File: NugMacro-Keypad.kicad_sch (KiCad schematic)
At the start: 16 parts, among them J2 Conn_01x04, SW1 SW_Push, U1 ATmega32U4-A, Y1 16MHz

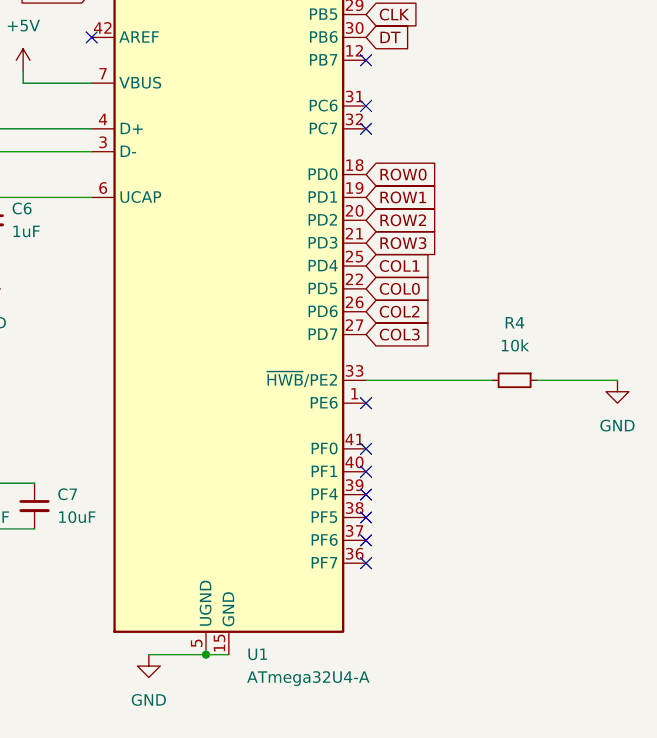
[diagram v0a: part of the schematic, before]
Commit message: First prototype pcb done
finally
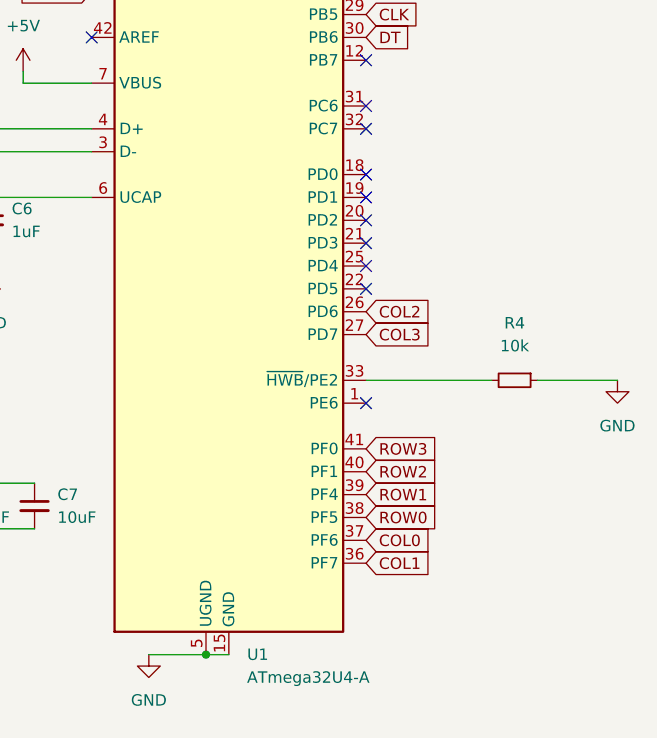
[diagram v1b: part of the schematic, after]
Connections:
- net COL0: now also U1.37 (PF6); no longer U1.22 (PD5)
- net COL1: now also U1.36 (PF7); no longer U1.25 (PD4)
- net ROW0: now also U1.38 (PF5); no longer U1.18 (PD0)
- net ROW1: now also U1.39 (PF4); no longer U1.19 (PD1)
- net ROW2: now also U1.40 (PF1); no longer U1.20 (PD2)
- net ROW3: now also U1.41 (PF0); no longer U1.21 (PD3)
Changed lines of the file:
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@@
   (no_connect (at 195.58 71.12))
   (no_connect (at 226.06 73.66))
-  (no_connect (at 226.06 124.46))
+  (no_connect (at 226.06 88.9))
+  (no_connect (at 226.06 86.36))
+  (no_connect (at 226.06 96.52))
   (no_connect (at 226.06 81.28))
-  (no_connect (at 226.06 119.38))
   (no_connect (at 226.06 111.76))
-  (no_connect (at 226.06 129.54))
   (no_connect (at 226.06 60.96))
+  (no_connect (at 226.06 93.98))
   (no_connect (at 226.06 63.5))
-  (no_connect (at 226.06 121.92))
-  (no_connect (at 226.06 127))
-  (no_connect (at 226.06 116.84))
+  (no_connect (at 226.06 91.44))
+  (no_connect (at 226.06 99.06))
   (no_connect (at 226.06 66.04))
   (no_connect (at 226.06 78.74))
@@
     )
   )
-  (global_label "ROW3" (shape input) (at 226.06 93.98 0) (fields_autoplaced)
-    (effects (font (size 1.27 1.27)) (justify left))
-    (property "Intersheet References" "${INTERSHEET_REFS}" (id 0) (at 233.7345 93.9006 0)
+  (global_label "ROW3" (shape input) (at 226.06 116.84 0) (fields_autoplaced)
+    (effects (font (size 1.27 1.27)) (justify left))
+    (property "Intersheet References" "${INTERSHEET_REFS}" (id 0) (at 233.7345 116.7606 0)
       (effects (font (size 1.27 1.27)) (justify left) hide)
     )
@@
     )
   )
-  (global_label "ROW0" (shape input) (at 226.06 86.36 0) (fields_autoplaced)
-    (effects (font (size 1.27 1.27)) (justify left))
-    (property "Intersheet References" "${INTERSHEET_REFS}" (id 0) (at 233.7345 86.2806 0)
+  (global_label "ROW0" (shape input) (at 226.06 124.46 0) (fields_autoplaced)
+    (effects (font (size 1.27 1.27)) (justify left))
+    (property "Intersheet References" "${INTERSHEET_REFS}" (id 0) (at 233.7345 124.3806 0)
       (effects (font (size 1.27 1.27)) (justify left) hide)
     )
@@
     )
   )
-  (global_label "COL0" (shape input) (at 226.06 99.06 0) (fields_autoplaced)
-    (effects (font (size 1.27 1.27)) (justify left))
-    (property "Intersheet References" "${INTERSHEET_REFS}" (id 0) (at 233.3112 98.9806 0)
+  (global_label "COL0" (shape input) (at 226.06 127 0) (fields_autoplaced)
+    (effects (font (size 1.27 1.27)) (justify left))
+    (property "Intersheet References" "${INTERSHEET_REFS}" (id 0) (at 233.3112 126.9206 0)
       (effects (font (size 1.27 1.27)) (justify left) hide)
     )
@@
     )
   )
-  (global_label "ROW1" (shape input) (at 226.06 88.9 0) (fields_autoplaced)
-    (effects (font (size 1.27 1.27)) (justify left))
-    (property "Intersheet References" "${INTERSHEET_REFS}" (id 0) (at 233.7345 88.8206 0)
+  (global_label "ROW1" (shape input) (at 226.06 121.92 0) (fields_autoplaced)
+    (effects (font (size 1.27 1.27)) (justify left))
+    (property "Intersheet References" "${INTERSHEET_REFS}" (id 0) (at 233.7345 121.8406 0)
       (effects (font (size 1.27 1.27)) (justify left) hide)
     )
@@
     )
   )
-  (global_label "COL1" (shape input) (at 226.06 96.52 0) (fields_autoplaced)
-    (effects (font (size 1.27 1.27)) (justify left))
-    (property "Intersheet References" "${INTERSHEET_REFS}" (id 0) (at 233.3112 96.4406 0)
+  (global_label "COL1" (shape input) (at 226.06 129.54 0) (fields_autoplaced)
+    (effects (font (size 1.27 1.27)) (justify left))
+    (property "Intersheet References" "${INTERSHEET_REFS}" (id 0) (at 233.3112 129.4606 0)
       (effects (font (size 1.27 1.27)) (justify left) hide)
     )
@@
     )
   )
-  (global_label "ROW2" (shape input) (at 226.06 91.44 0) (fields_autoplaced)
-    (effects (font (size 1.27 1.27)) (justify left))
-    (property "Intersheet References" "${INTERSHEET_REFS}" (id 0) (at 233.7345 91.3606 0)
-      (effects (font (size 1.27 1.27)) (justify left) hide)
-    )
+  (global_label "ROW2" (shape input) (at 226.06 119.38 0) (fields_autoplaced)
+    (effects (font (size 1.27 1.27)) (justify left))
+    (property "Intersheet References" "${INTERSHEET_REFS}" (id 0) (at 233.7345 119.3006 0)
+      (effects (font (size 1.27 1.27)) (justify left) hide)
+    )

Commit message: its done
yay
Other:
- company: MIT Liscence -> MIT License
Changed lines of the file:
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@@
     (title "Nug Macro V3")
     (rev "V3")
-    (company "MIT Liscence")
+    (company "MIT License")
   )
   (junction (at 88.9 111.76) (diameter 0) (color 0 0 0 0)
